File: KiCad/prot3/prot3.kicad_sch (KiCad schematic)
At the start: 201 parts, among them J1 Conn_01x02_Socket, J2 LED_SW, J3 Conn_01x04_Socket, Q1 Q_Photo_NPN, Q10 Q_Photo_NPN, Q11 Q_Photo_NPN, Q12 Q_Photo_NPN, Q13 Q_Photo_NPN, Q14 Q_Photo_NPN, Q15 Q_Photo_NPN, Q16 Q_Photo_NPN, Q17 Q_Photo_NPN, Q18 Q_Photo_NPN, Q19 Q_Photo_NPN, Q2 Q_Photo_NPN, Q20 Q_Photo_NPN, Q21 Q_Photo_NPN, Q22 Q_Photo_NPN, Q23 Q_Photo_NPN, Q24 Q_Photo_NPN, Q25 Q_Photo_NPN, Q26 Q_Photo_NPN, Q27 Q_Photo_NPN, Q28 Q_Photo_NPN, Q29 Q_Photo_NPN, Q3 Q_Photo_NPN, Q30 Q_Photo_NPN, Q31 Q_Photo_NPN, Q32 Q_Photo_NPN, Q4 Q_Photo_NPN, Q5 Q_Photo_NPN, Q6 Q_Photo_NPN, Q7 Q_Photo_NPN, Q8 Q_Photo_NPN, Q9 Q_Photo_NPN, U1 LM339, U2 LM339, U3 LM339, U4 LM339, U5 LM339, U6 LM339, U7 LM339, U8 LM339

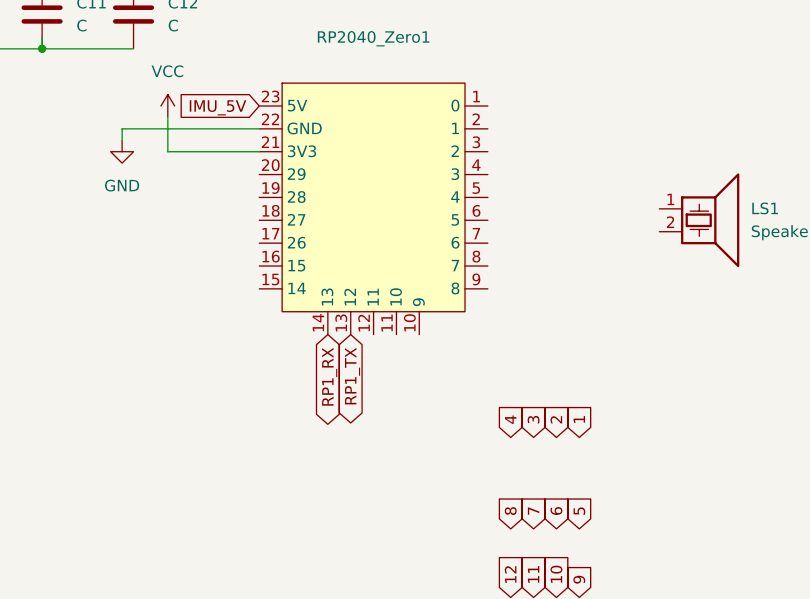
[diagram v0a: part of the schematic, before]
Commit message: バイブコーディングはうんこ
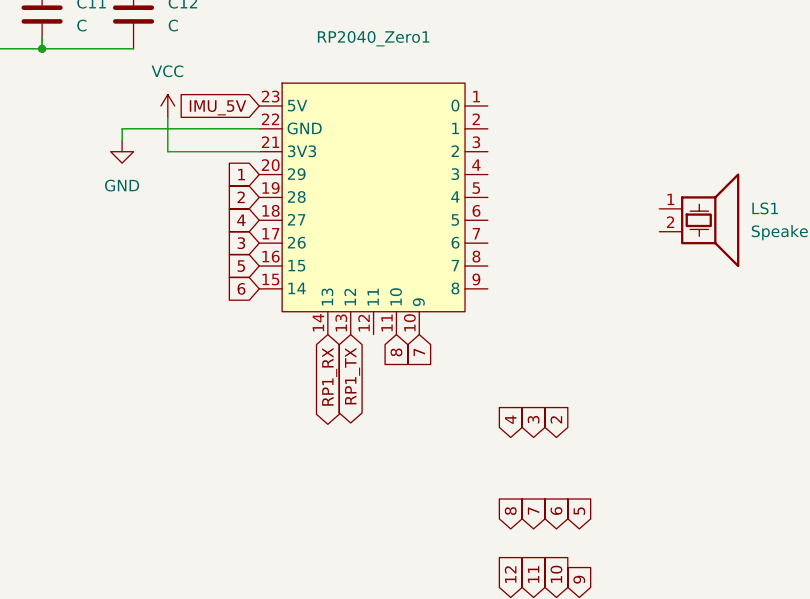
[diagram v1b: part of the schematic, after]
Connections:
- net 1: now also RP2040_Zero1.20 (29)
- net 2: now also RP2040_Zero1.19 (28)
- net 3: now also RP2040_Zero1.17 (26)
- net 4: now also RP2040_Zero1.18 (27)
- net 5: now also RP2040_Zero1.16 (15)
- net 6: now also RP2040_Zero1.15 (14)
- net 7: now also RP2040_Zero1.10 (9)
- net 8: now also RP2040_Zero1.11 (10)
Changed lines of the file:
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@@
 		)
 	)
+	(global_label "8"
+		(shape input)
+		(at 102.87 312.42 270)
+		(fields_autoplaced yes)
+		(effects
+			(font
+				(size 1.27 1.27)
+			)
+			(justify right)
+		)
+		(property "Intersheetrefs" "${INTERSHEET_REFS}"
+			(at 102.87 316.6147 90)
+			(effects
+				(font
+					(size 1.27 1.27)
+				)
+				(justify right)
+				(hide yes)
+			)
+		)
+	)
 	(global_label "LED_5V"
 		(shape input)
@@
 		)
 	)
+	(global_label "6"
+		(shape input)
+		(at 87.63 307.34 180)
+		(fields_autoplaced yes)
+		(effects
+			(font
+				(size 1.27 1.27)
+			)
+			(justify right)
+		)
+		(property "Intersheetrefs" "${INTERSHEET_REFS}"
+			(at 83.4353 307.34 0)
+			(effects
+				(font
+					(size 1.27 1.27)
+				)
+				(justify right)
+				(hide yes)
+			)
+		)
+	)
 	(global_label "conp_+"
 		(shape bidirectional)
@@
 		)
 	)
+	(global_label "4"
+		(shape input)
+		(at 87.63 299.72 180)
+		(fields_autoplaced yes)
+		(effects
+			(font
+				(size 1.27 1.27)
+			)
+			(justify right)
+		)
+		(property "Intersheetrefs" "${INTERSHEET_REFS}"
+			(at 83.4353 299.72 0)
+			(effects
+				(font
+					(size 1.27 1.27)
+				)
+				(justify right)
+				(hide yes)
+			)
+		)
+	)
 	(global_label "2B"
 		(shape input)
@@
 	(global_label "7"
 		(shape input)
+		(at 105.41 312.42 270)
+		(fields_autoplaced yes)
+		(effects
+			(font
+				(size 1.27 1.27)
+			)
+			(justify right)
+		)
+		(property "Intersheetrefs" "${INTERSHEET_REFS}"
+			(at 105.41 316.6147 90)
+			(effects
+				(font
+					(size 1.27 1.27)
+				)
+				(justify right)
+				(hide yes)
+			)
+		)
+	)
+	(global_label "7"
+		(shape input)
 		(at 647.7 256.54 90)
 		(fields_autoplaced yes)
@@
 		)
 	)
+	(global_label "2"
+		(shape input)
+		(at 87.63 297.18 180)
+		(fields_autoplaced yes)
+		(effects
+			(font
+				(size 1.27 1.27)
+			)
+			(justify right)
+		)
+		(property "Intersheetrefs" "${INTERSHEET_REFS}"
+			(at 83.4353 297.18 0)
+			(effects
+				(font
+					(size 1.27 1.27)
+				)
+				(justify right)
+				(hide yes)
+			)
+		)
+	)
 	(global_label "IMU_5V"
 		(shape input)
@@
 		)
 	)
+	(global_label "3"
+		(shape input)
+		(at 87.63 302.26 180)
+		(fields_autoplaced yes)
+		(effects
+			(font
+				(size 1.27 1.27)
+			)
+			(justify right)
+		)
+		(property "Intersheetrefs" "${INTERSHEET_REFS}"
+			(at 83.4353 302.26 0)
+			(effects
+				(font
+					(size 1.27 1.27)
+				)
+				(justify right)
+				(hide yes)
+			)
+		)
+	)
 	(global_label "5D"
 		(shape input)
@@
 	(global_label "1"
 		(shape input)
-		(at 123.19 323.85 90)
+		(at 87.63 294.64 180)
 		(fields_autoplaced yes)
 		(effects
@@
 				(size 1.27 1.27)
 			)
-			(justify left)
+			(justify right)
 		)
 		(property "Intersheetrefs" "${INTERSHEET_REFS}"
-			(at 123.19 319.6553 90)
+			(at 83.4353 294.64 0)
 			(effects
 				(font
 					(size 1.27 1.27)
 				)
-				(justify left)
+				(justify right)
 				(hide yes)
 			)
@@
 				(hide yes)
 			)
+		)
+	)
+	(global_label "5"
+		(shape input)
+		(at 87.63 304.8 180)
+		(fields_autoplaced yes)
+		(effects
+			(font
+				(size 1.27 1.27)
+			)
+			(justify right)
+		)
+		(property "Intersheetrefs" "${INTERSHEET_REFS}"
+			(at 83.4353 304.8 0)
+			(effects
+				(font
+					(size 1.27 1.27)
+				)
+				(justify right)
+				(hide yes)
+			)
